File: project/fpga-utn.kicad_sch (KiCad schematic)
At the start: 0 parts

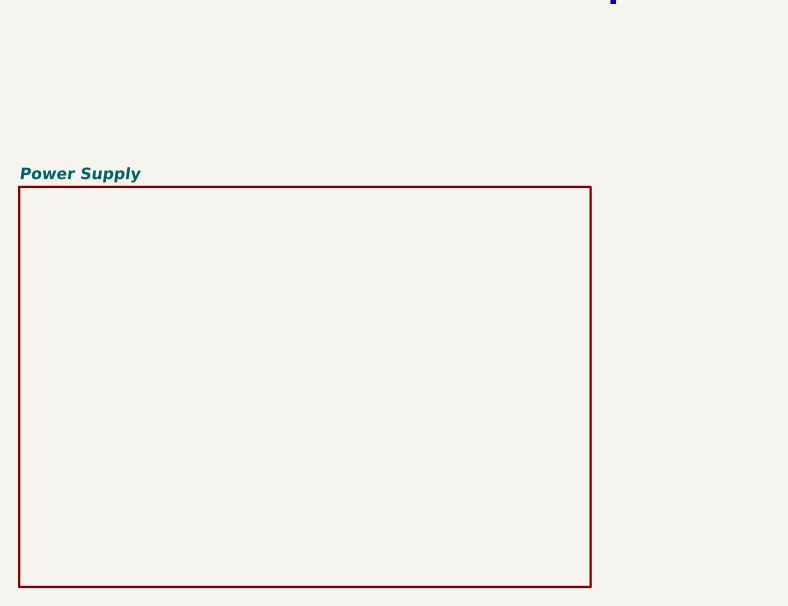
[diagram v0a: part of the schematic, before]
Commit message: Regulador V1 finalizado
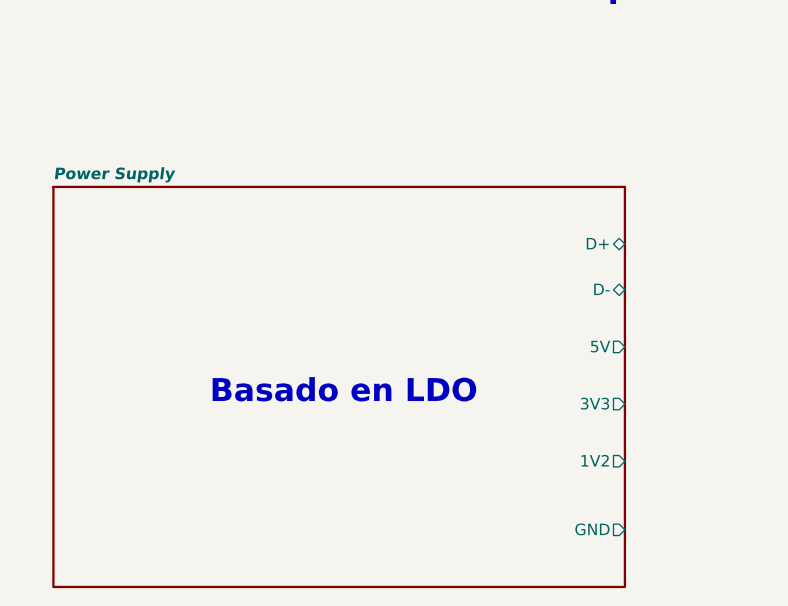
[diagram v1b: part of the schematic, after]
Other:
- sheet Power Supply ports: added 1V2, 3V3, 5V, D+, D-, GND; removed none
- note added: "Basado en LDO"
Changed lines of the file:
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@@
 	(generator_version "8.0")
 	(paper "A4")
+	(text "Basado en LDO"
+		(exclude_from_sim no)
+		(at 66.548 69.85 0)
+		(effects
+			(font
+				(size 2.55 2.55)
+				(thickness 0.51)
+				(bold yes)
+			)
+		)
+	)
 	(text "Aqui se inicia nuestro proyecto final"
 		(exclude_from_sim no)
@@
 	)
 	(sheet
-		(at 30.48 46.99)
+		(at 34.29 46.99)
 		(size 63.5 44.45)
 		(stroke
@@
 		)
 		(property "Sheetname" "Power Supply"
-			(at 30.48 46.2784 0)
+			(at 34.29 46.2784 0)
 			(effects
 				(font
@@
 		)
 		(property "Sheetfile" "power_supply.kicad_sch"
-			(at 30.48 92.0246 0)
+			(at 34.29 92.0246 0)
 			(effects
 				(font
@@
 			)
 		)
+		(pin "D+" bidirectional
+			(at 97.79 53.34 0)
+			(effects
+				(font
+					(size 1.27 1.27)
+				)
+				(justify right)
+			)
+		)
+		(pin "D-" bidirectional
+			(at 97.79 58.42 0)
+			(effects
+				(font
+					(size 1.27 1.27)
+				)
+				(justify right)
+			)
+		)
+		(pin "1V2" output
+			(at 97.79 77.47 0)
+			(effects
+				(font
+					(size 1.27 1.27)
+				)
+				(justify right)
+			)
+		)
+		(pin "3V3" output
+			(at 97.79 71.12 0)
+			(effects
+				(font
+					(size 1.27 1.27)
+				)
+				(justify right)
+			)
+		)
+		(pin "GND" output
+			(at 97.79 85.09 0)
+			(effects
+				(font
+					(size 1.27 1.27)
+				)
+				(justify right)
+			)
+		)
+		(pin "5V" output
+			(at 97.79 64.77 0)
+			(effects
+				(font
+					(size 1.27 1.27)
+				)
+				(justify right)
+			)
+		)
